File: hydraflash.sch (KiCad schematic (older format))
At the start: 10 parts, among them J1 CONN_02X07, J2 CONN_02X10, J3 CONN_02X10, J4 CONN_01X06, P1 WRITE_PROTECT, U1 Flash_NAND

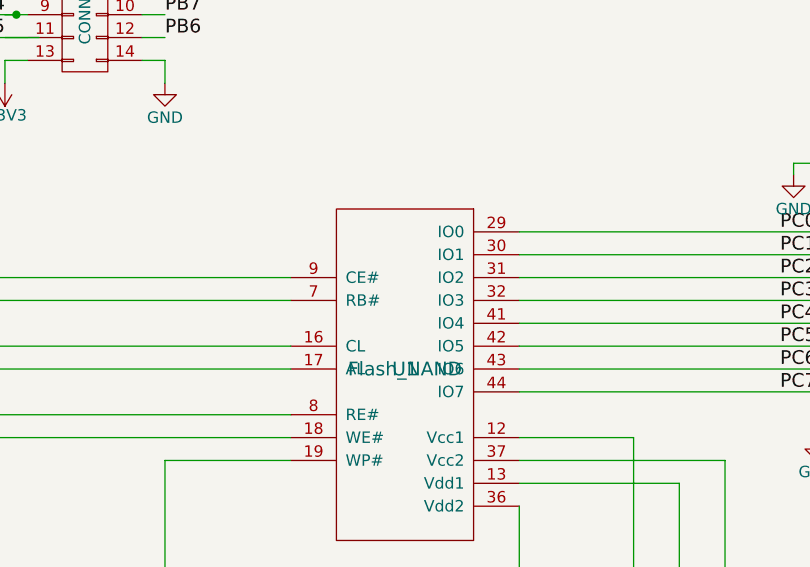
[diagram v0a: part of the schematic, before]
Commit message: Routing improvements by bvernoux
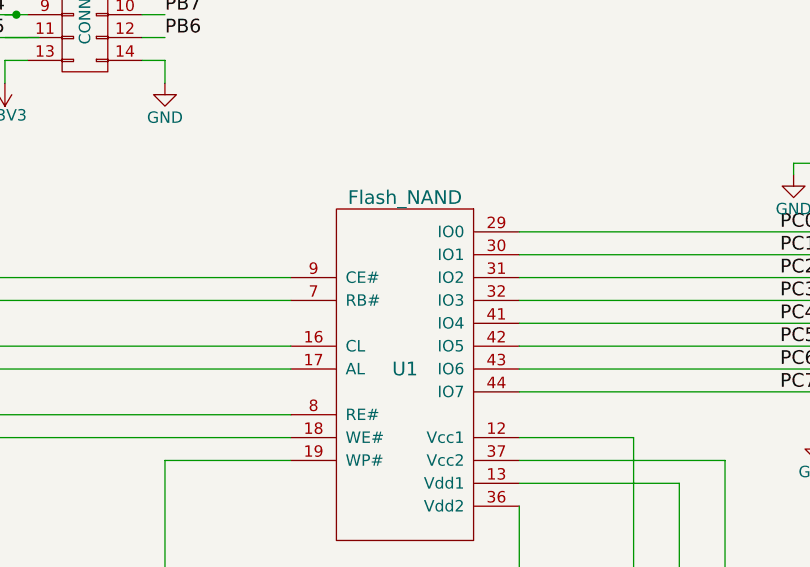
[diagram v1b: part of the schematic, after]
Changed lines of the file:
@@
 LIBS:contrib
 LIBS:valves
-LIBS:hydrabus-shield-template-cache
+LIBS:hydraflash-cache
 EELAYER 25 0
 EELAYER END
@@
 P 5250 3750
 F 0 "U1" H 5250 3750 60  0000 C CNN
-F 1 "Flash_NAND" H 5250 3750 60  0000 C CNN
+F 1 "Flash_NAND" H 5250 4500 60  0000 C CNN
 F 2 "tsop48_socket:TSOP48ZIF" H 5250 3750 60  0001 C CNN
 F 3 "" H 5250 3750 60  0000 C CNN
